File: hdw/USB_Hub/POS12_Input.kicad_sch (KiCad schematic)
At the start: 21 parts, among them J201 +12V IN, U201 TPS26600RHFT

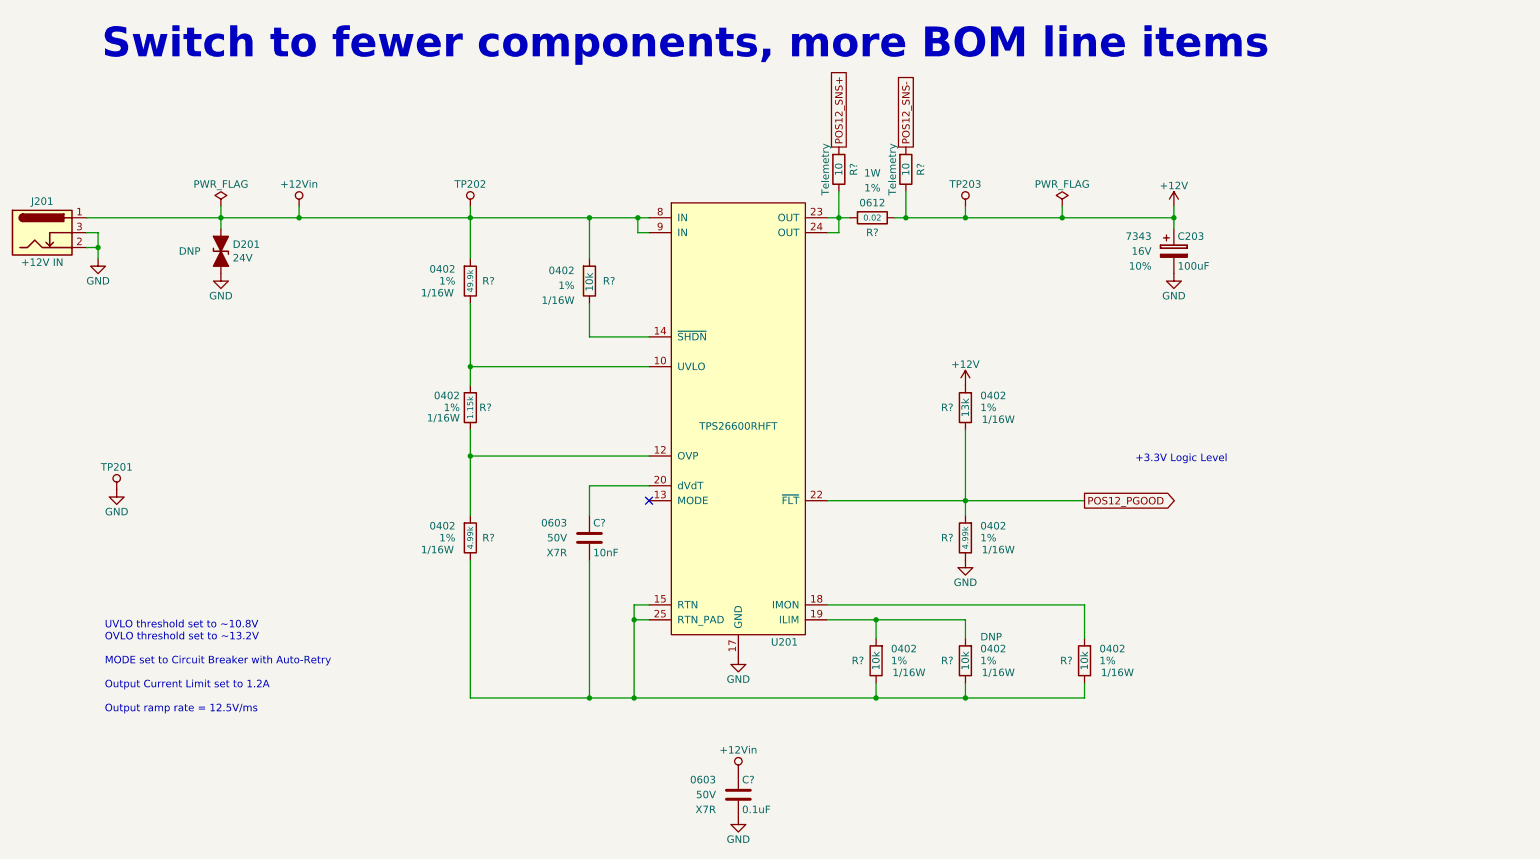
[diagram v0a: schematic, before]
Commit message: much more schematic progress
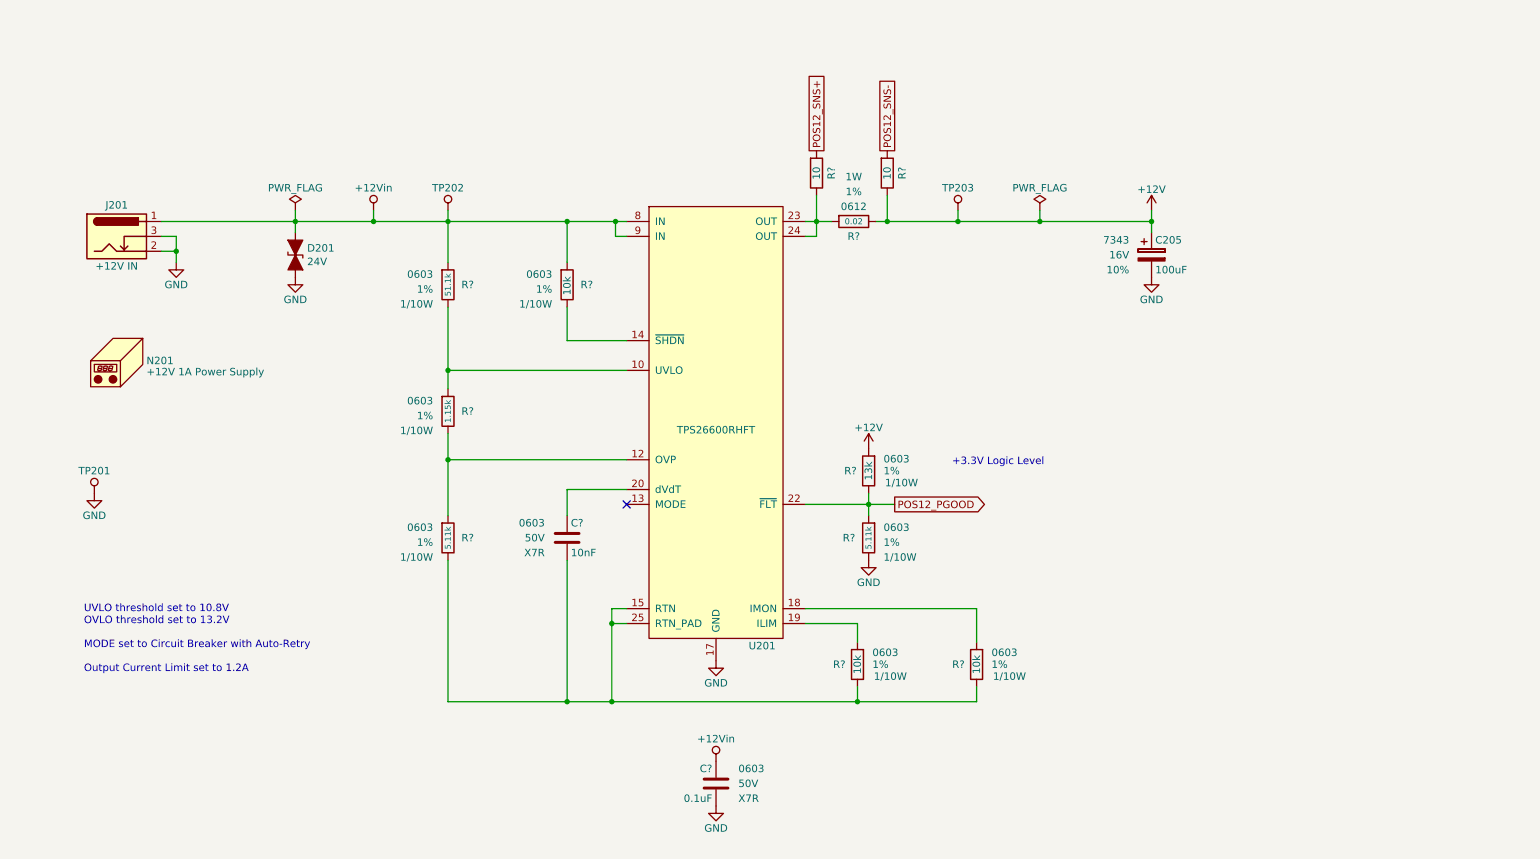
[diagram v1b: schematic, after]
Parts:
- removed C203: 100uF, Capacitors_Tantalum_SMD:CP_Tantalum_Case-X_EIA-7343-43_Reflow, symbol Custom_Library:CP_Tant_Custom
- removed C?: 0.1uF, Capacitors_SMD:C_0603, symbol Custom_Library:C_Custom
- removed C?: 10nF, Capacitors_SMD:C_0603, symbol Custom_Library:C_Custom
- removed R? (x2): 4.99k, Resistors_SMD:R_0402, symbol Custom_Library:R_Custom
- removed R? (x4): 10k, Resistors_SMD:R_0402, symbol Custom_Library:R_Custom
- removed R? (x2): 10, Resistors_SMD:R_0402, symbol Custom_Library:R_Custom
- removed R?: 1.15k, Resistors_SMD:R_0402, symbol Custom_Library:R_Custom
- removed R?: 0.02, Resistors_SMD:R_0612, symbol Custom_Library:R_Custom
- removed R?: 13k, Resistors_SMD:R_0402, symbol Custom_Library:R_Custom
- removed R?: 49.9k, Resistors_SMD:R_0402, symbol Custom_Library:R_Custom
- added C205: 100uF, Capacitors_Tantalum_SMD:CP_Tantalum_Case-X_EIA-7343-43_Reflow, symbol Custom_Library:CP_Tant_Custom
- added C?: 10nF, Capacitors_SMD:C_0603, symbol Custom_Library:C_Custom
- added C?: 0.1uF, Capacitors_SMD:C_0603, symbol Custom_Library:C_Custom
- added N201: +12V 1A Power Supply, symbol Mechanical:Housing
- added R? (x2): 10, Resistors_SMD:R_0603, symbol Custom_Library:R_Custom
- added R? (x3): 10k, Resistors_SMD:R_0603, symbol Custom_Library:R_Custom
- added R?: 1.15k, Resistors_SMD:R_0603, symbol Custom_Library:R_Custom
- added R?: 13k, Resistors_SMD:R_0603, symbol Custom_Library:R_Custom
- added R? (x2): 5.11k, Resistors_SMD:R_0603, symbol Custom_Library:R_Custom
- added R?: 51.1k, Resistors_SMD:R_0603, symbol Custom_Library:R_Custom
- added R?: 0.02, Resistors_SMD:R_0612, symbol Custom_Library:R_Custom
- D201: Configuration DNP -> (none)
- TP202, TP203: value TP -> TP_Pad
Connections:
- net +12V: now also C205.1, R?.1, R?.2, R?.2
- net +12Vin: now also C?.1, R?.1, R?.1
- net GND: now also C205.2, C?.2, R?.2
- net POS12_PGOOD: now also R?.1, R?.2
- net POS12_SNS+: now also R?.1
- net POS12_SNS-: now also R?.1
- net at U201.14 (~{SHDN}): now also R?.2
- net at U201.12 (OVP): now also R?.1, R?.2
- net at U201.15 (RTN), U201.25 (RTN_PAD): now also C?.2, R?.2, R?.2, R?.2
- net at U201.10 (UVLO): now also R?.1, R?.2
- net at U201.18 (IMON): now also R?.1
- net at U201.19 (ILIM): now also R?.1
- net at U201.20 (dVdT): now also C?.1
- net at U201.23 (OUT), U201.24 (OUT): now also R?.1, R?.2
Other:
- note added: "UVLO threshold set to 10.8V OVLO threshold set to 13.2V MODE set to Circuit Breaker with Auto-Retry Output Current Limit set to 1.2A"
- note removed: "Switch to fewer components, more BOM line items"
- note removed: "UVLO threshold set to ~10.8V OVLO threshold set to ~13.2V MODE set to Circuit Breaker with Auto-Retry Output Current Limit set to 1.2A Output ramp rate = 12.5V/ms"
